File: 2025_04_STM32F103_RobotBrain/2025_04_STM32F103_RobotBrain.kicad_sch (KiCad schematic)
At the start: 25 parts, among them J1 USB_B_Mini, SW1 SW_SPST, U1 STM32F103RCTx, U2 USBLC6-2SC6, Y2 16Mhz

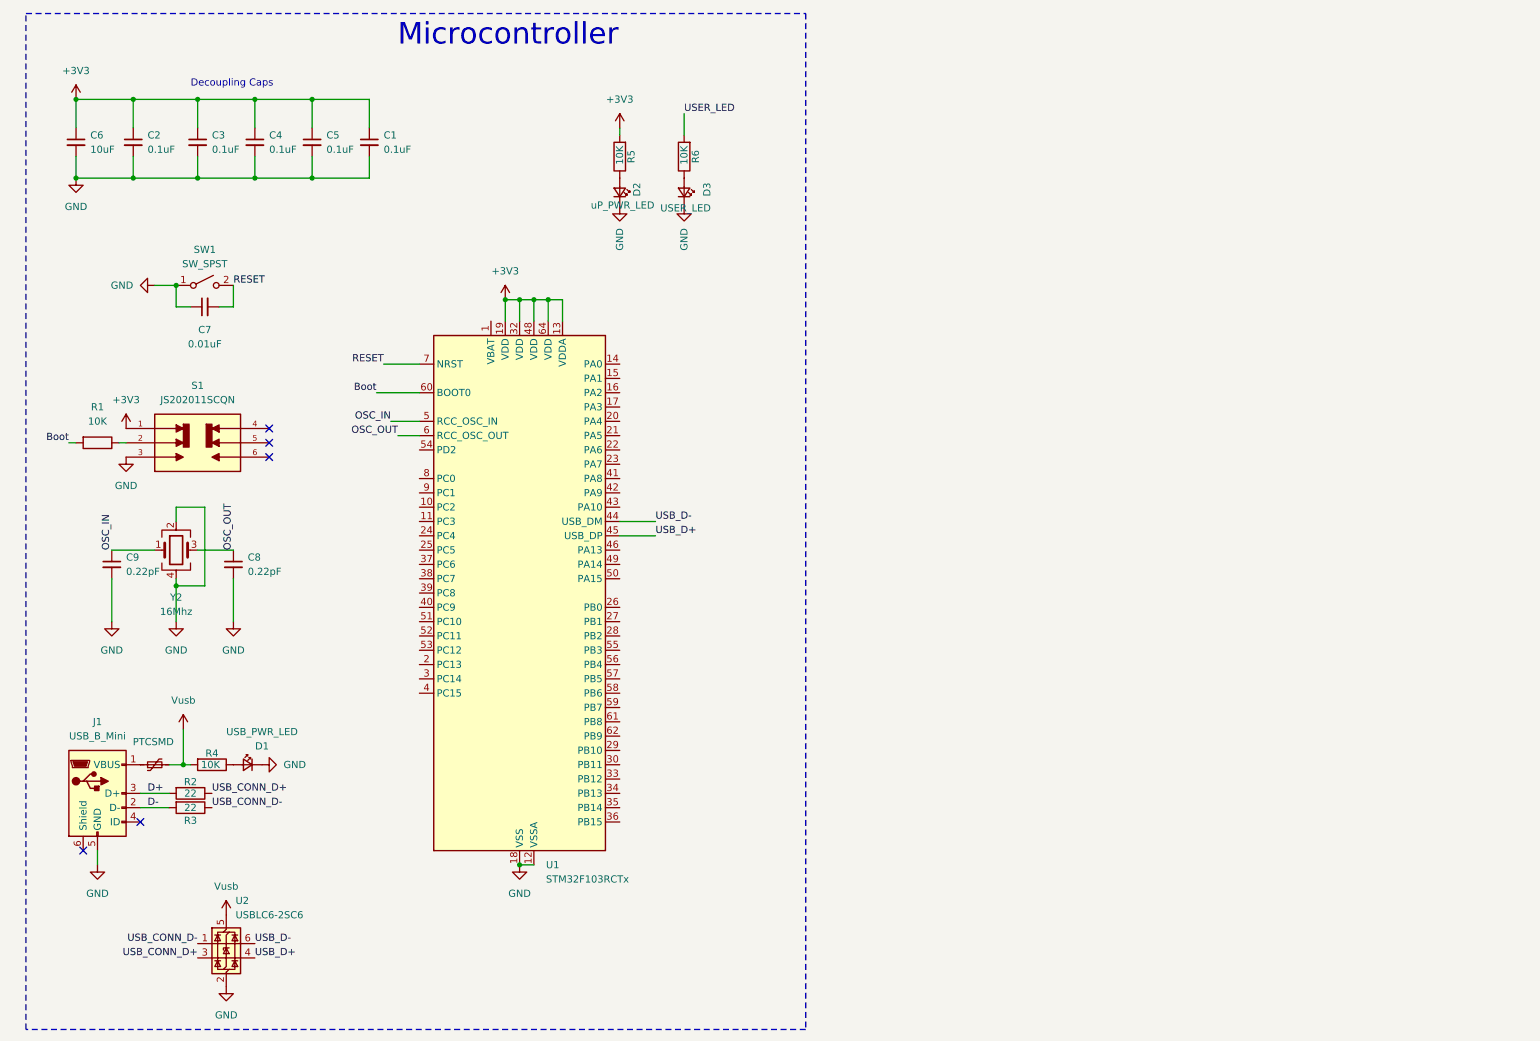
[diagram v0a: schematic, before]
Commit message: Robotbrain
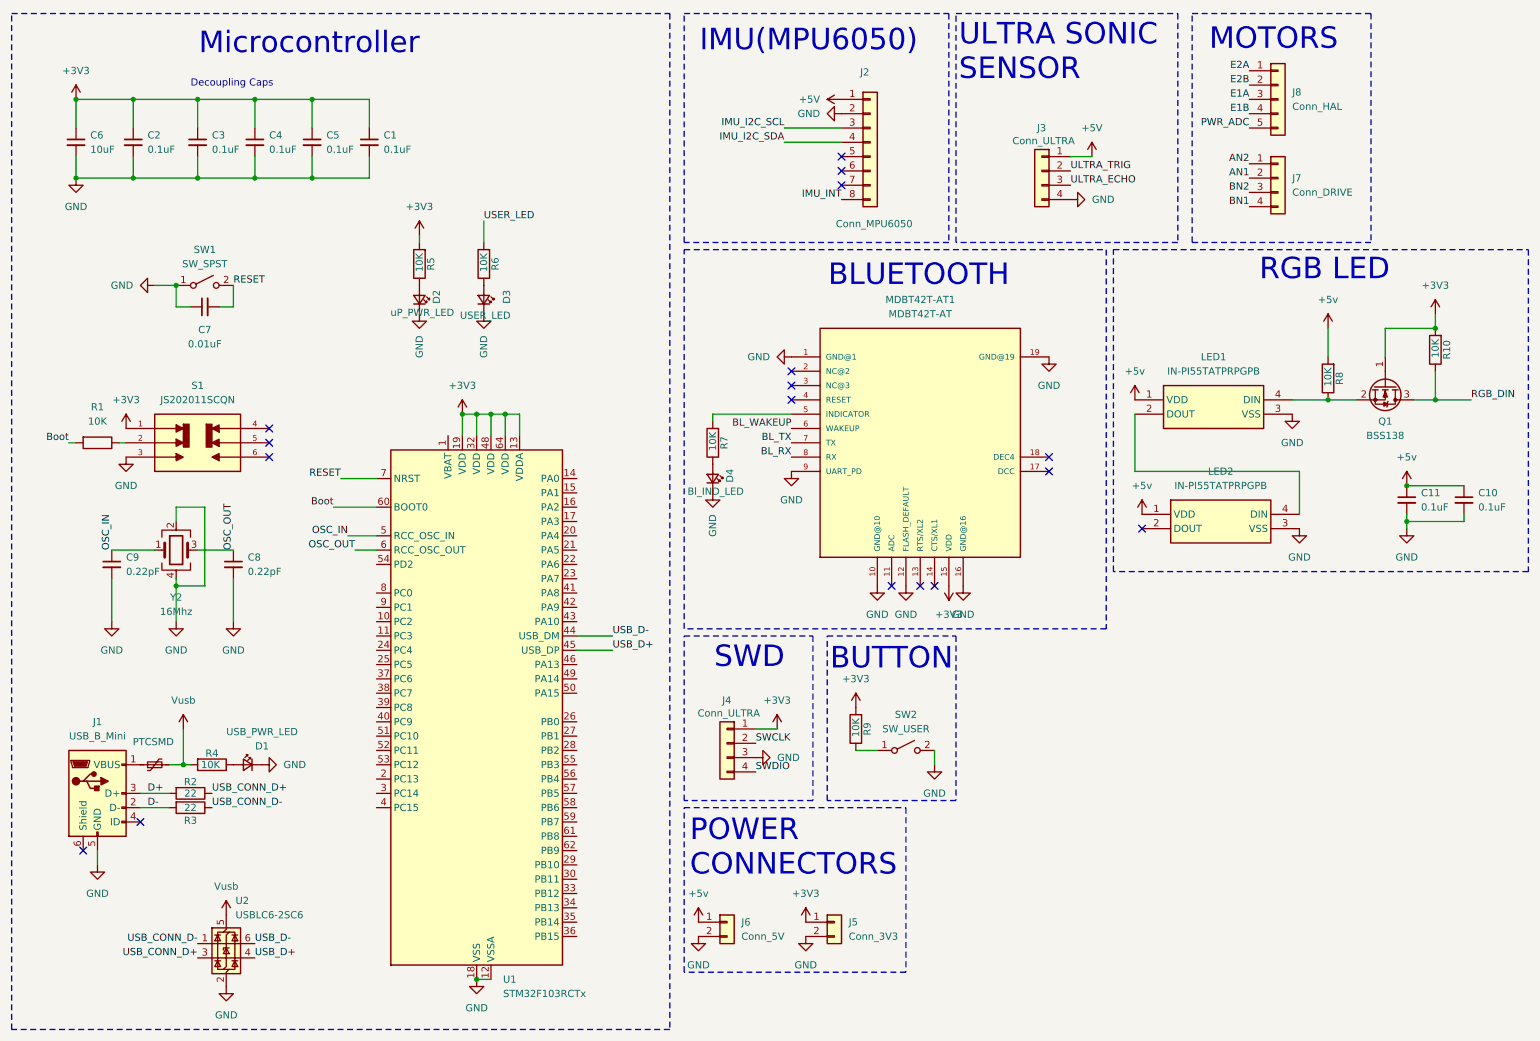
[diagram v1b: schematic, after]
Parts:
- added C10, C11: 0.1uF, Capacitor_SMD:C_0805_2012Metric_Pad1.18x1.45mm_HandSolder, symbol Device:C_Small
- added D4: Bl_IND_LED, LED_SMD:LED_0805_2012Metric, symbol Device:LED_Small
- added J2: Conn_MPU6050, Connector_PinHeader_2.54mm:PinHeader_1x08_P2.54mm_Vertical, symbol Connector_Generic:Conn_01x08
- added J3, J4: Conn_ULTRA, Connector_PinHeader_2.54mm:PinHeader_1x04_P2.54mm_Vertical, symbol Connector_Generic:Conn_01x04
- added J5: Conn_3V3, Connector_JST:JST_XH_B2B-XH-A_1x02_P2.50mm_Vertical, symbol Connector_Generic:Conn_01x02
- added J6: Conn_5V, Connector_JST:JST_XH_B2B-XH-A_1x02_P2.50mm_Vertical, symbol Connector_Generic:Conn_01x02
- added J7: Conn_DRIVE, Connector_JST:JST_XH_B4B-XH-A_1x04_P2.50mm_Vertical, symbol Connector_Generic:Conn_01x04
- added J8: Conn_HAL, Connector_JST:JST_XH_B5B-XH-A_1x05_P2.50mm_Vertical, symbol Connector_Generic:Conn_01x05
- added LED1, LED2: IN-PI55TATPRPGPB, RGB_LED:INPI55TATPRPGPB, symbol RGB_LED:IN-PI55TATPRPGPB
- added MDBT42T-AT1: MDBT42T-AT, MDBT42T-AT:MDBT42T, symbol MDBT42T-AT:MDBT42T-AT
- added Q1: BSS138, Package_TO_SOT_SMD:SOT-23, symbol Transistor_FET:BSS138
- added R10, R7, R8, R9: 10K, Resistor_SMD:R_0805_2012Metric_Pad1.20x1.40mm_HandSolder, symbol Device:R
- added SW2: SW_USER, Button_Switch_SMD:SW_SPST_PTS647_Sx50, symbol Switch:SW_SPST
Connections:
- net +3V3: now also J4.1 (Pin_1), J5.1 (Pin_1), MDBT42T-AT1.15 (VDD), Q1.1 (G), R10.2, R9.2
- net GND: now also C10.2, C11.2, D4.1 (K), J2.2 (Pin_2), J3.4 (Pin_4), J4.3 (Pin_3), J5.2 (Pin_2), J6.2 (Pin_2), LED1.3 (VSS), LED2.3 (VSS), MDBT42T-AT1.1 (GND@1), MDBT42T-AT1.10 (GND@10), MDBT42T-AT1.12 (FLASH_DEFAULT), MDBT42T-AT1.16 (GND@16), MDBT42T-AT1.19 (GND@19), MDBT42T-AT1.9 (UART_PD), SW2.2 (B)
- new net: LED1.2 (DOUT), LED2.4 (DIN)
- new net: LED1.4 (DIN), Q1.2 (S), R8.1
- new net: MDBT42T-AT1.5 (INDICATOR), R7.2
- new net: R9.1, SW2.1 (A)
- new net: D4.2 (A), R7.1
- new net +5V: J2.1 (Pin_1), J3.1 (Pin_1)
- new net +5v: C10.1, C11.1, J6.1 (Pin_1), LED1.1 (VDD), LED2.1 (VDD), R8.2
- new net AN1: J7.2 (Pin_2)
- new net AN2: J7.1 (Pin_1)
- new net BL_RX: MDBT42T-AT1.8 (RX)
- new net BL_TX: MDBT42T-AT1.7 (TX)
- new net BL_WAKEUP: MDBT42T-AT1.6 (WAKEUP)
- new net BN1: J7.4 (Pin_4)
- new net BN2: J7.3 (Pin_3)
- new net E1A: J8.3 (Pin_3)
- new net E1B: J8.4 (Pin_4)
- new net E2A: J8.1 (Pin_1)
- new net E2B: J8.2 (Pin_2)
- new net IMU_I2C_SCL: J2.3 (Pin_3)
- new net IMU_I2C_SDA: J2.4 (Pin_4)
- new net IMU_INT: J2.8 (Pin_8)
- new net PWR_ADC: J8.5 (Pin_5)
- new net RGB_DIN: Q1.3 (D), R10.1
- new net SWCLK: J4.2 (Pin_2)
- new net SWDIO: J4.4 (Pin_4)
- new net ULTRA_ECHO: J3.3 (Pin_3)
- new net ULTRA_TRIG: J3.2 (Pin_2)
- no-connect marks 5 -> 17
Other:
- note added: "BLUETOOTH"
- note added: "BUTTON"
- note added: "IMU(MPU6050)"
- note added: "MOTORS"
- note added: "POWER CONNECTORS"
- note added: "RGB LED"
- note added: "SWD"
- note added: "ULTRA SONIC SENSOR"
- moved on the sheet: D2, D3, R5, R6, U1
